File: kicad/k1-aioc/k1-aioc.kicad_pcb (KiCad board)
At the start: 4 copper layers, 21 x 31.5 mm, 72 parts, among them J1 12401832E402A, J3 FT817-CAT, J4 FT817-CAT, J5 USB, J6 Conn_ARM_SWD_TagConnect_TC203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, Q1 MMBT3904, Q3 MMBT3904, Q4 MMBT3904, U1 MIC5330-SSYML, U2 STM32F373CBTx, Y1 8MHz/20pF

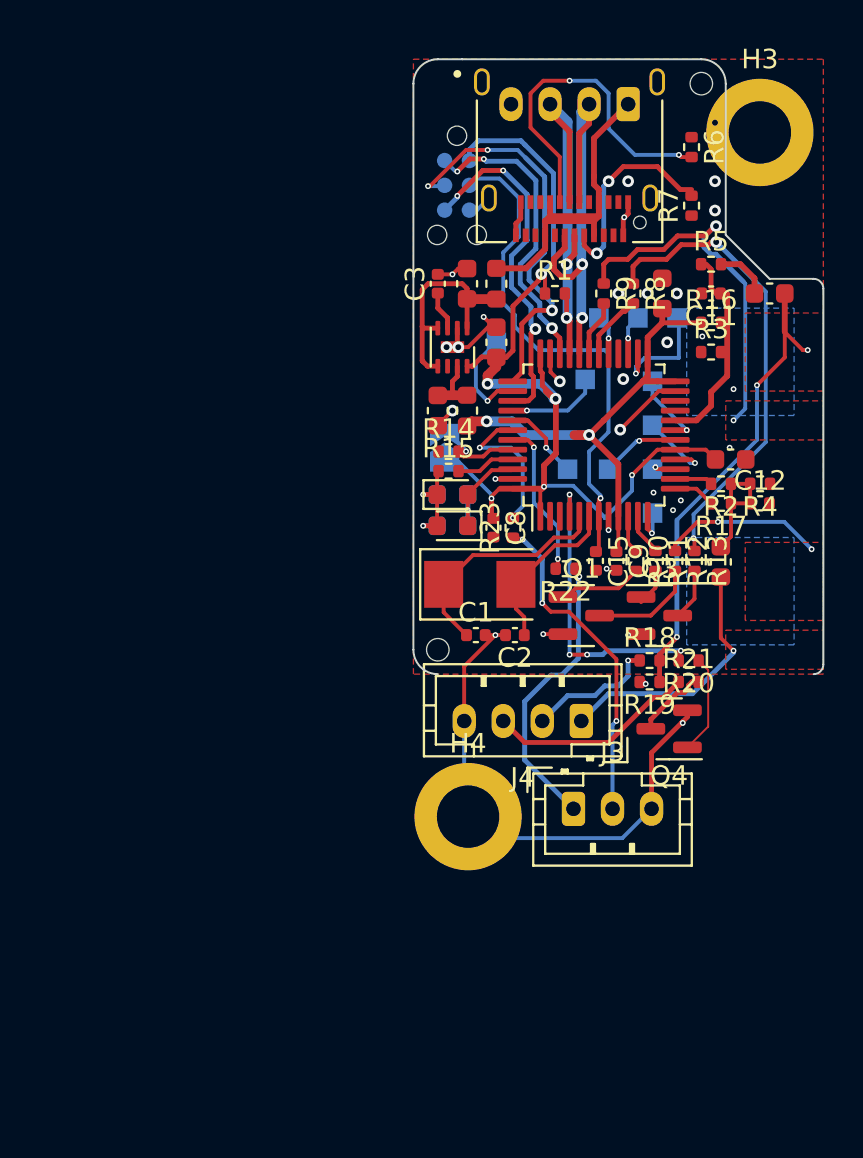
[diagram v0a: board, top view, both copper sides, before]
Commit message: Commit before assembly
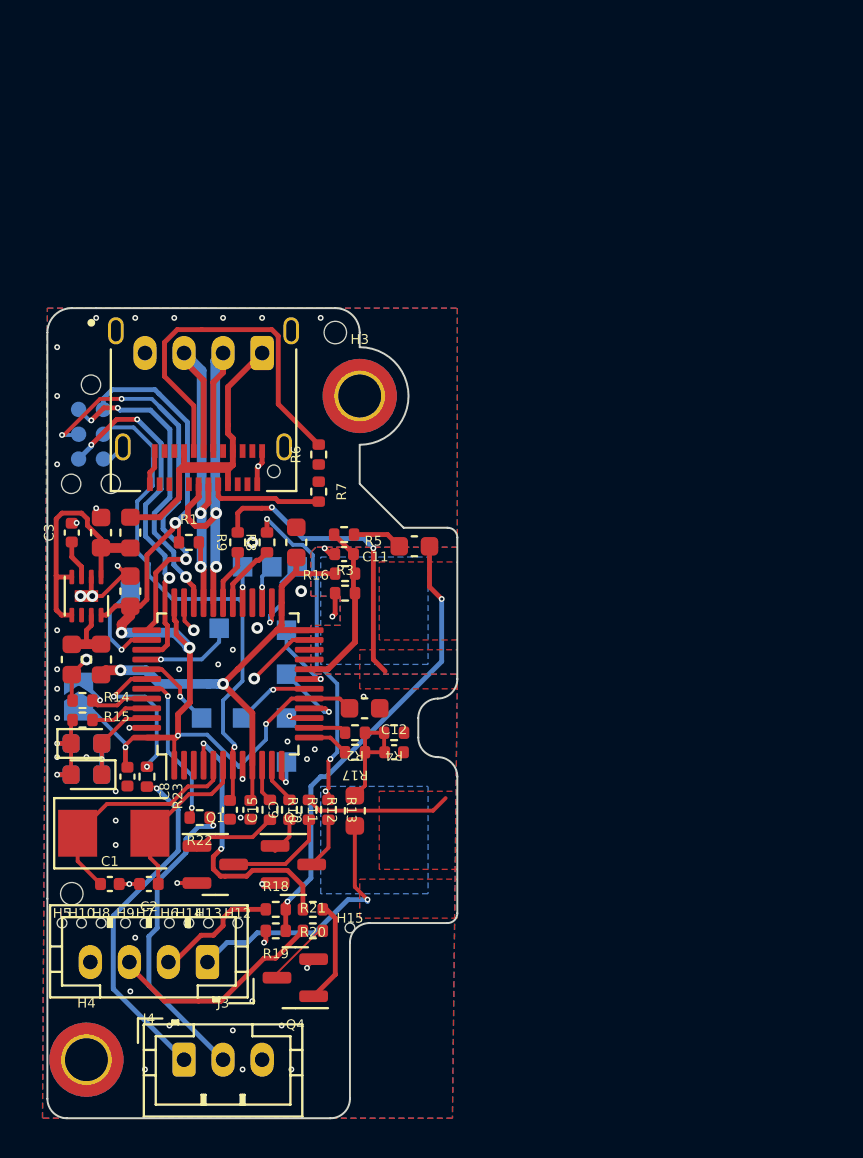
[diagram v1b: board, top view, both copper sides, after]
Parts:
- added H10: Breakaway Hole, AIOC:breakawayHole, F.Cu at (86.5, 124.2)
- added H12: Breakaway Hole, AIOC:breakawayHole, F.Cu at (94.5, 124.2)
- added H13: Breakaway Hole, AIOC:breakawayHole, F.Cu at (93.0, 124.2)
- added H14: Breakaway Hole, AIOC:breakawayHole, F.Cu at (92.0, 124.2)
- added H15: Breakaway Hole, AIOC:breakawayHole, F.Cu at (100.2, 124.5)
- added H5: Breakaway Hole, AIOC:breakawayHole, F.Cu at (85.5, 124.2)
- added H6: Breakaway Hole, AIOC:breakawayHole, F.Cu at (91.0, 124.2)
- added H7: Breakaway Hole, AIOC:breakawayHole, F.Cu at (89.8, 124.2)
- added H8: Breakaway Hole, AIOC:breakawayHole, F.Cu at (87.5, 124.2)
- added H9: Breakaway Hole, AIOC:breakawayHole, F.Cu at (88.8, 124.2)
- H3, H4: footprint MountingHole:MountingHole_3.2mm_M3_ISO14580_Pad -> MountingHole:MountingHole_2.2mm_M2_ISO14580_Pad_TopBottom
- moved REF** 36.1 mm to (91.8, 118.2)
- moved R6 24.8 mm to (98.7, 100.2), turned to 90 degrees
- moved H3 24.5 mm to (100.8, 97.2)
- moved R7 24.1 mm to (98.7, 102.2), turned to -90 degrees
- moved J3 23.7 mm to (91.8, 131.2)
- moved R5 23.4 mm to (100.0, 104.3)
- moved TP11 23.3 mm to (97.5, 106.0)
- moved H4 23.2 mm to (86.8, 131.2)
- moved R20 23.1 mm to (98.3, 123.5)
- moved R21 23.1 mm to (98.3, 124.7)
- moved C11 23.1 mm to (100.0, 105.3)
- moved Q4 23.0 mm to (97.5, 127.0)
- moved R18 23.0 mm to (96.5, 123.5)
- moved R19 23.0 mm to (96.5, 124.7)
- moved J4 22.8 mm to (93.0, 126.2)
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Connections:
- R22 pad 1: Net-(J3-Pin_1) -> Net-(J3-Pin_2)
- R23 pad 1: Net-(J3-Pin_2) -> Net-(J3-Pin_1)
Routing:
- net GND: track 47.7 -> 24.9 mm, vias 31 -> 56
- net /RADIO-RX-PTT1: track 24.1 -> 17.4 mm, vias 2 -> 3
- net Net-(J1-CC1): track 10.1 -> 5.87 mm, vias 2 -> 0
- net /RADIO-TX: track 19.1 -> 15.5 mm
- net Net-(J3-Pin_1): track 14.9 -> 17.8 mm
- net /AFIN: track 10.5 -> 8.88 mm
- net /VIN: track 11.5 -> 13.0 mm
- net Net-(J1-CC2): track 17.4 -> 18.8 mm, vias 2 -> 0
- net Net-(U2-PB14): track 5.88 -> 4.48 mm
- net Net-(J3-Pin_2): track 17.0 -> 15.8 mm, vias 3 -> 1
- net /817_PTT: track 15.6 -> 14.5 mm, vias 4 -> 2
- net /RADIO-VP-PTT2: track 8.39 -> 7.49 mm, vias 2 -> 0
- net +3V3: track 53.5 -> 52.8 mm
- net Net-(U2-PA8): track 2.04 -> 1.34 mm
- net /RADIO-SPK: track 24.0 -> 23.4 mm, vias 3 -> 2
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- added copper zone on In2.Cu, net GND
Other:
- board size 21 x 31.5 mm -> 21 x 41.5 mm
- board text added: "AIOC V1.2"
- board text added: "AUD AUD PTT GND OUT IN OUT"
- board text added: "GND D+ D- +5"
- board text added: "GND SER SER OUT IN"
- board text added: "S. Kueppers AB1TJ"
- board text removed: "AIOC V1.0"
- board text removed: "S. Kueppers"
- board text removed: "SWD"
